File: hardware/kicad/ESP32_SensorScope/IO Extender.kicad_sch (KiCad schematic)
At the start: 0 parts

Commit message: som updates on the schematics
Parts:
- added U25: TCA9535PWR, Package_SO:TSSOP-24_4.4x7.8mm_P0.65mm, symbol Interface_Expansion:TCA9535PWR
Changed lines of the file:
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@@
 	(generator_version "8.0")
 	(paper "A4")
+	(global_label "IO_INT"
+		(shape input)
+		(at 67.31 73.66 180)
+		(fields_autoplaced yes)
+		(effects
+			(font
+				(size 1.27 1.27)
+			)
+			(justify right)
+		)
+		(property "Intersheetrefs" "${INTERSHEET_REFS}"
+			(at 58.519 73.66 0)
+			(effects
+				(font
+					(size 1.27 1.27)
+				)
+				(justify right)
+			)
+		)
+	)
+	(symbol
+		(lib_id "Interface_Expansion:TCA9535PWR")
+		(at 87.63 88.9 0)
+		(unit 1)
+		(exclude_from_sim no)
+		(in_bom yes)
+		(on_board yes)
+		(dnp no)
+		(fields_autoplaced yes)
+		(property "Reference" "U25"
+			(at 89.8241 60.96 0)
+			(effects
+				(font
+					(size 1.27 1.27)
+				)
+				(justify left)
+			)
+		)
+		(property "Value" "TCA9535PWR"
+			(at 89.8241 63.5 0)
+			(effects
+				(font
+					(size 1.27 1.27)
+				)
+				(justify left)
+			)
+		)
+		(property "Footprint" "Package_SO:TSSOP-24_4.4x7.8mm_P0.65mm"
+			(at 114.3 114.3 0)
+			(effects
+				(font
+					(size 1.27 1.27)
+				)
+				(hide yes)
+			)
+		)
+		(property "Datasheet" "http://www.ti.com/lit/ds/symlink/tca9535.pdf"
+			(at 74.93 66.04 0)
+			(effects
+				(font
+					(size 1.27 1.27)
+				)
+				(hide yes)
+			)
+		)
+		(property "Description" "16-bit I/O expander, I2C and SMBus interface, interrupts, w/o pull-ups, TSSOP-24 package"
+			(at 87.63 88.9 0)
+			(effects
+				(font
+					(size 1.27 1.27)
+				)
+				(hide yes)
+			)
+		)
+		(pin "1"
+		)
+		(pin "17"
+		)
+		(pin "14"
+		)
+		(pin "3"
+		)
+		(pin "13"
+		)
+		(pin "20"
+		)
+		(pin "5"
+		)
+		(pin "15"
+		)
+		(pin "2"
+		)
+		(pin "23"
+		)
+		(pin "18"
+		)
+		(pin "8"
+		)
+		(pin "16"
+		)
+		(pin "12"
+		)
+		(pin "19"
+		)
+		(pin "11"
+		)
+		(pin "21"
+		)
+		(pin "22"
+		)
+		(pin "4"
+		)
+		(pin "24"
+		)
+		(pin "10"
+		)
+		(pin "7"
+		)
+		(pin "9"
+		)
+		(pin "6"
+		)
+		(instances
+			(project ""
+				(path "/53b18f60-802b-4114-ad1b-2672cfed64a1/46b88311-9688-470c-917a-6dd4762a83c9"
+					(reference "U25")
+					(unit 1)
+				)
+			)
+		)
+	)
 )

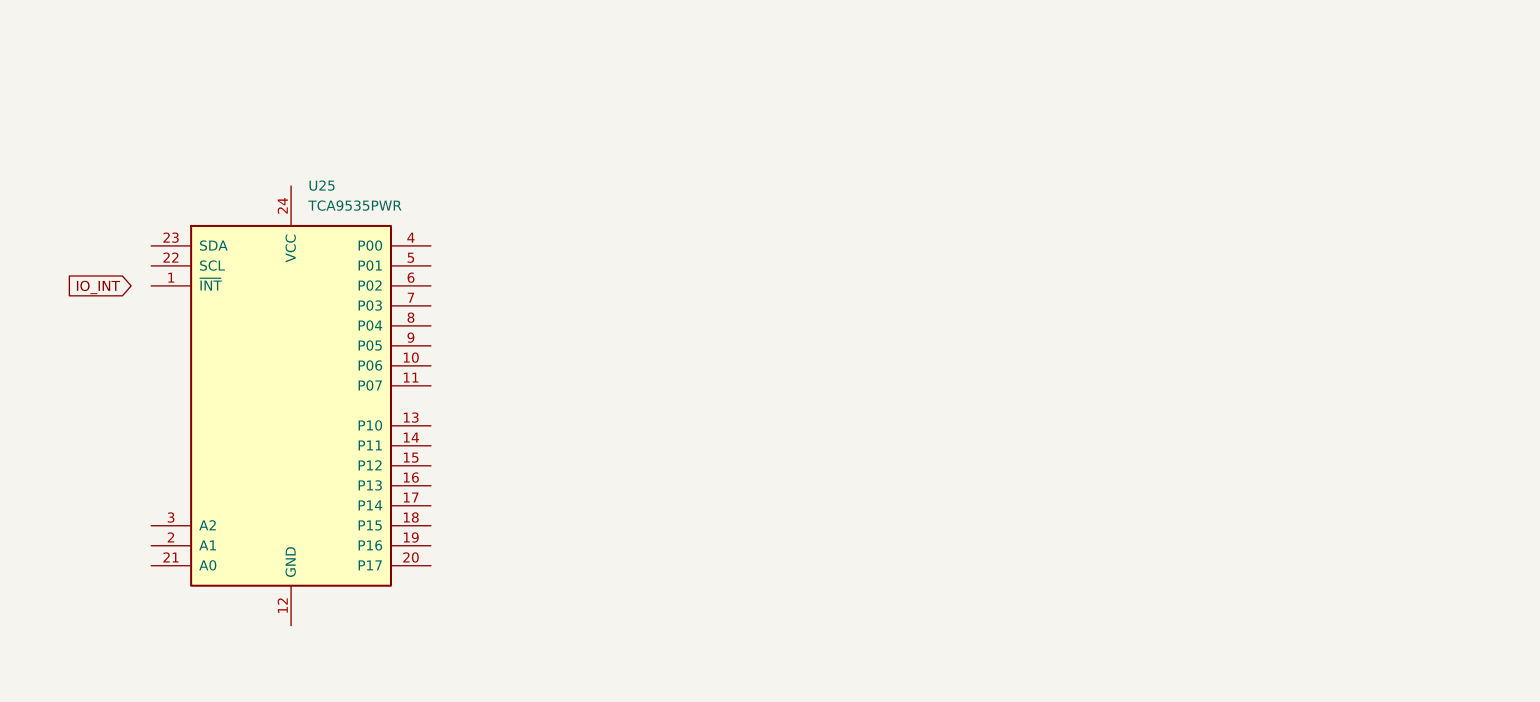
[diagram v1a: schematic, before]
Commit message: updatet schematic
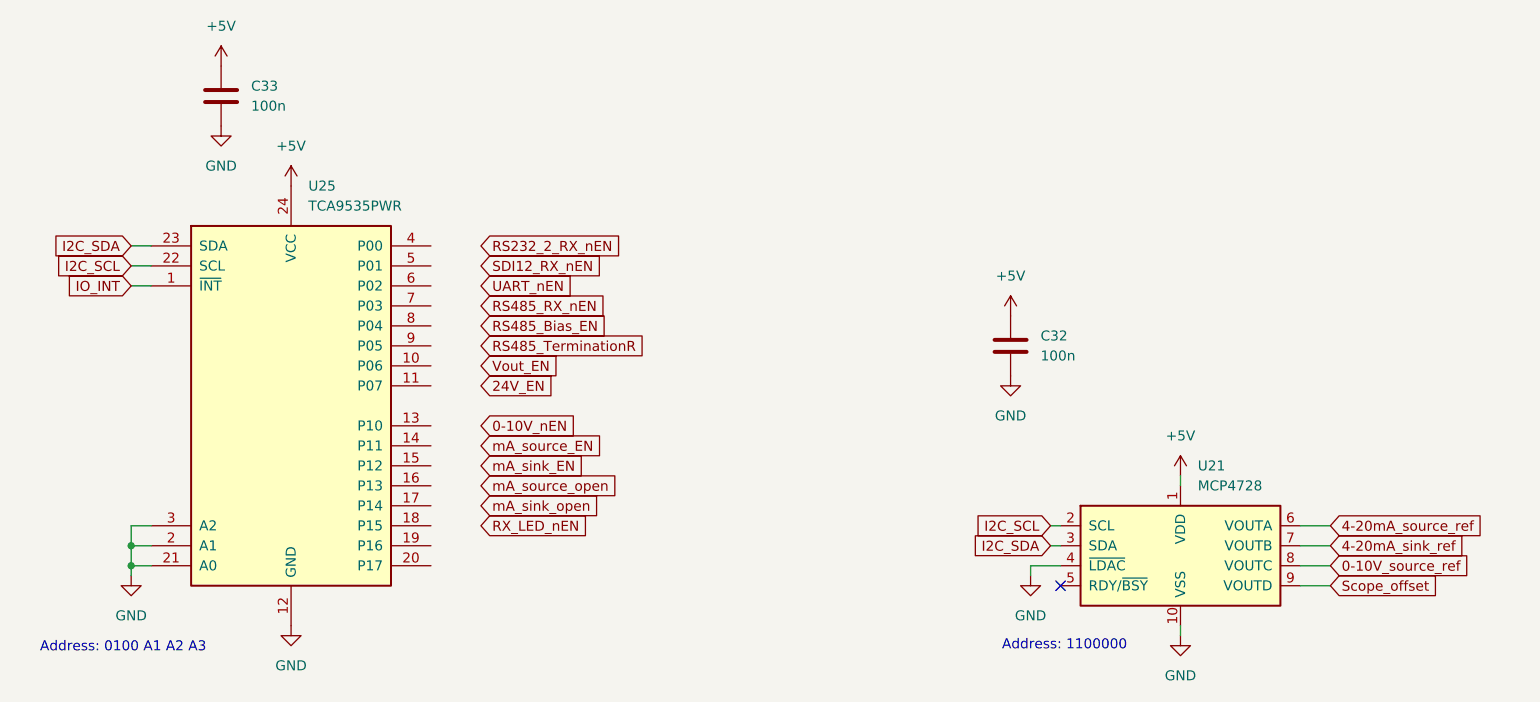
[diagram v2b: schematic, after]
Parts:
- added C32, C33: 100n, symbol Device:C
- added U21: MCP4728, Package_SO:MSOP-10_3x3mm_P0.5mm, symbol Analog_DAC:MCP4728
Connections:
- net IO_INT: now also U25.1 (~{INT})
- net GND: now reaches U25.12 (GND)
- net GND: now also U25.2 (A1), U25.21 (A0), U25.3 (A2), C32.2, C33.2, U21.10 (VSS), U21.4 (~{LDAC})
- net I2C_SCL: now reaches U25.22 (SCL)
- net I2C_SCL: now also U21.2 (SCL)
- net I2C_SDA: now reaches U25.23 (SDA)
- net I2C_SDA: now also U21.3 (SDA)
- net +5V: now reaches U25.24 (VCC)
- net +5V: now also C32.1, C33.1, U21.1 (VDD)
- new net 0-10V_source_ref: U21.8 (VOUTC)
- new net 4-20mA_sink_ref: U21.7 (VOUTB)
- new net 4-20mA_source_ref: U21.6 (VOUTA)
- new net Scope_offset: U21.9 (VOUTD)
- no-connect marks 0 -> 1
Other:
- note added: "Address: 0100 A1 A2 A3"
- note added: "Address: 1100000"

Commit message: addet some footprints"
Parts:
- C32, C33: footprint (none) -> Capacitor_SMD:C_0805_2012Metric
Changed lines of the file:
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@@
 			)
 		)
-		(property "Footprint" ""
+		(property "Footprint" "Capacitor_SMD:C_0805_2012Metric"
 			(at 79.7052 53.34 0)
 			(effects
@@
 			)
 		)
-		(property "Footprint" ""
+		(property "Footprint" "Capacitor_SMD:C_0805_2012Metric"
 			(at 180.0352 85.09 0)
 			(effects
